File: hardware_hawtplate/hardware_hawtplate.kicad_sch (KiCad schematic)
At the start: 36 parts, among them J1 Conn_01x02_Socket_XT60, J2 USB_C_Receptacle_USB2.0_16P, J3 Conn_01x04_Pin, Q1 AO3400A, SW1 SW_Push, SW2 SW_Push, SW3 SW_Push, U1 RP2040, U2 AMS1117-3.3, U3 W25Q16JVSS, Y1 Crystal_GND24

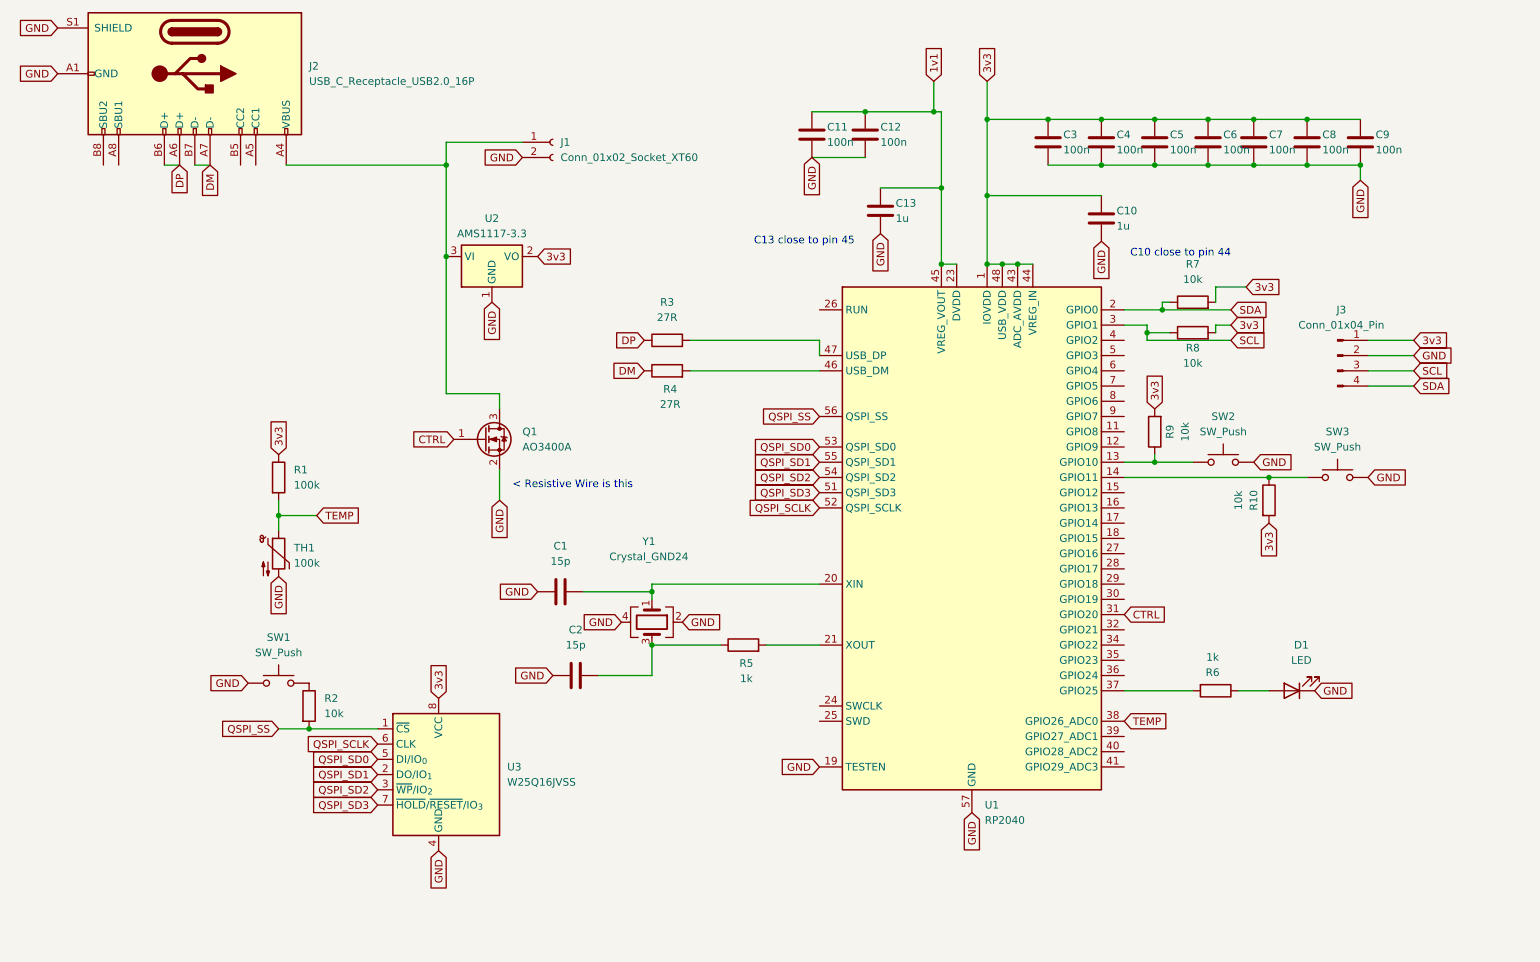
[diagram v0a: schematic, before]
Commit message: Schematic
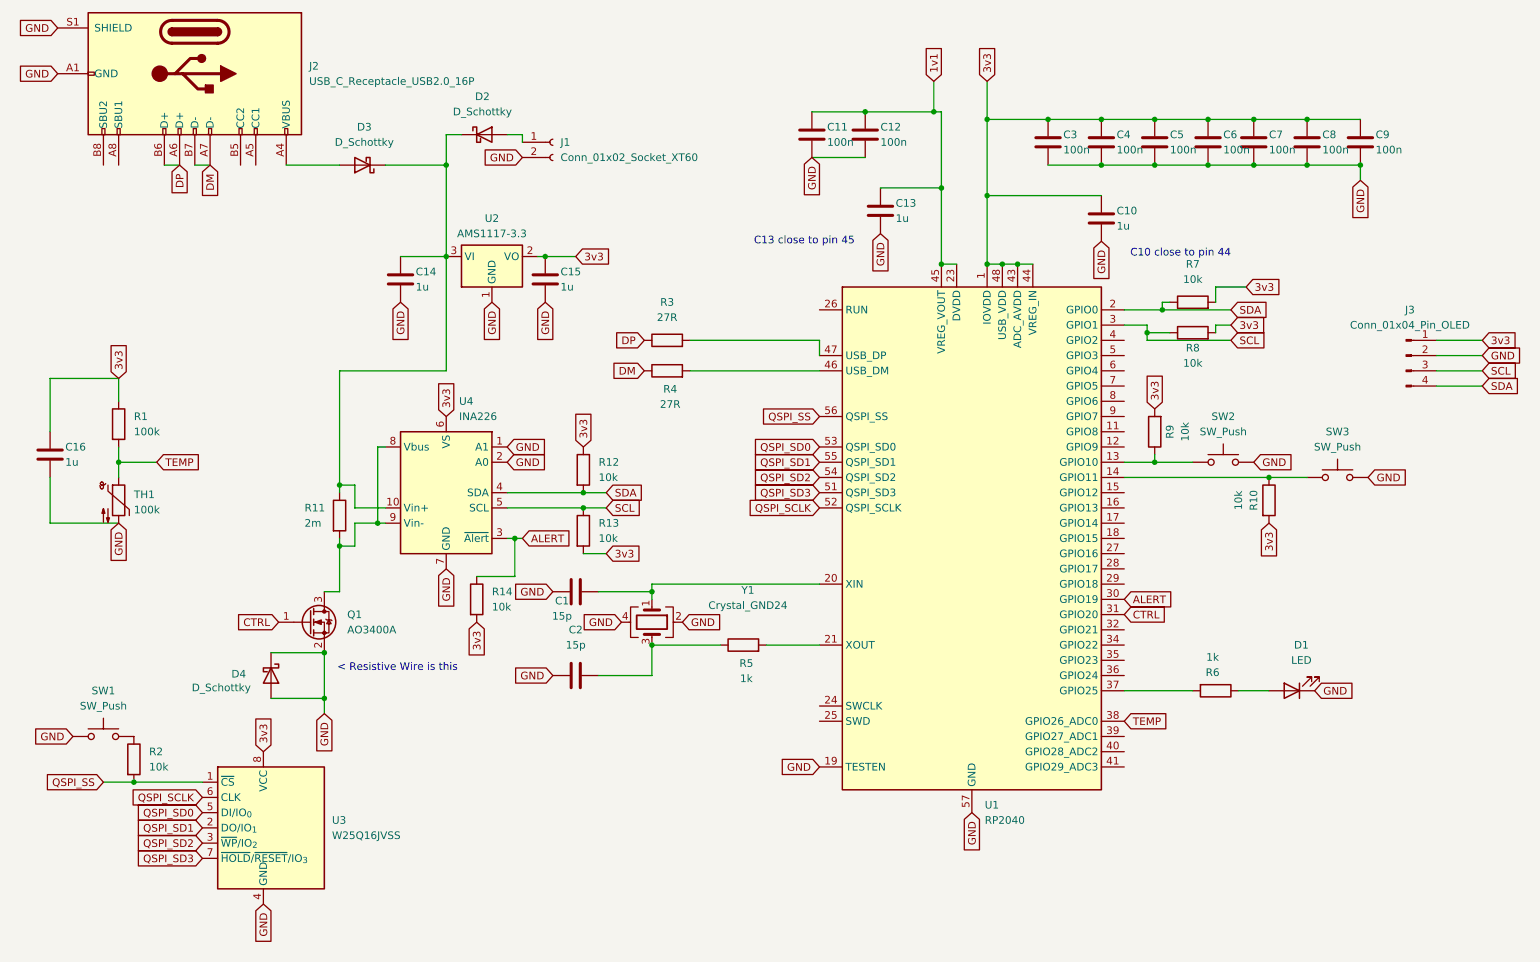
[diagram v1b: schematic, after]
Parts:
- added C14, C15, C16: 1u, Capacitor_SMD:C_0402_1005Metric, symbol Device:C
- added D2, D3, D4: D_Schottky, symbol Device:D_Schottky
- added R11: 2m, symbol Device:R
- added R12, R13, R14: 10k, symbol Device:R
- added U4: INA226, Package_SO:VSSOP-10_3x3mm_P0.5mm, symbol Sensor_Energy:INA226
- C1, C10, C11, C12, C13, C2, C3, C4, C5, C6, C7, C8, C9: footprint (none) -> Capacitor_SMD:C_0402_1005Metric
- D1: footprint (none) -> LED_SMD:LED_0402_1005Metric
- J1: footprint (none) -> Connector_PinHeader_2.54mm:PinHeader_1x01_P2.54mm_Vertical
- J3: value Conn_01x04_Pin -> Conn_01x04_Pin_OLED
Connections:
- net 3v3: now also C15.2, C16.2, R12.1, R13.2, R14.2, U4.6 (VS)
- net GND: now also C14.1, C15.1, C16.1, D4.1 (K), D4.2 (A), U4.1 (A1), U4.2 (A0), U4.7 (GND)
- net SCL: now also R13.1, U4.5 (SCL)
- net SDA: now also R12.2, U4.4 (SDA)
- net at J2.A4 (VBUS), J2.A9 (VBUS), J2.B4 (VBUS)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: now also D3.2 (A); no longer J1.1 (Pin_1), Q1.3 (D), U2.3 (VI)
- net ALERT: now reaches U1.30 (GPIO19)
- net ALERT: now also R14.1, U4.3 (~{Alert})
- new net: D2.2 (A), J1.1 (Pin_1)
- new net: C14.2, D2.1 (K), D3.1 (K), R11.1, U2.3 (VI), U4.10 (Vin+)
- new net: Q1.3 (D), R11.2, U4.8 (Vbus), U4.9 (Vin-)
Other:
- moved on the sheet: C1, J3, Q1, R1, R2, SW1, TH1, U3
